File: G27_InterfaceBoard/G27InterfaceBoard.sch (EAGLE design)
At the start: 28 parts, among them IC1 LMV321M5, IC2 74HC126D, J1 Pedal, J2 Shifter, J3 Steering, U1 LMV324

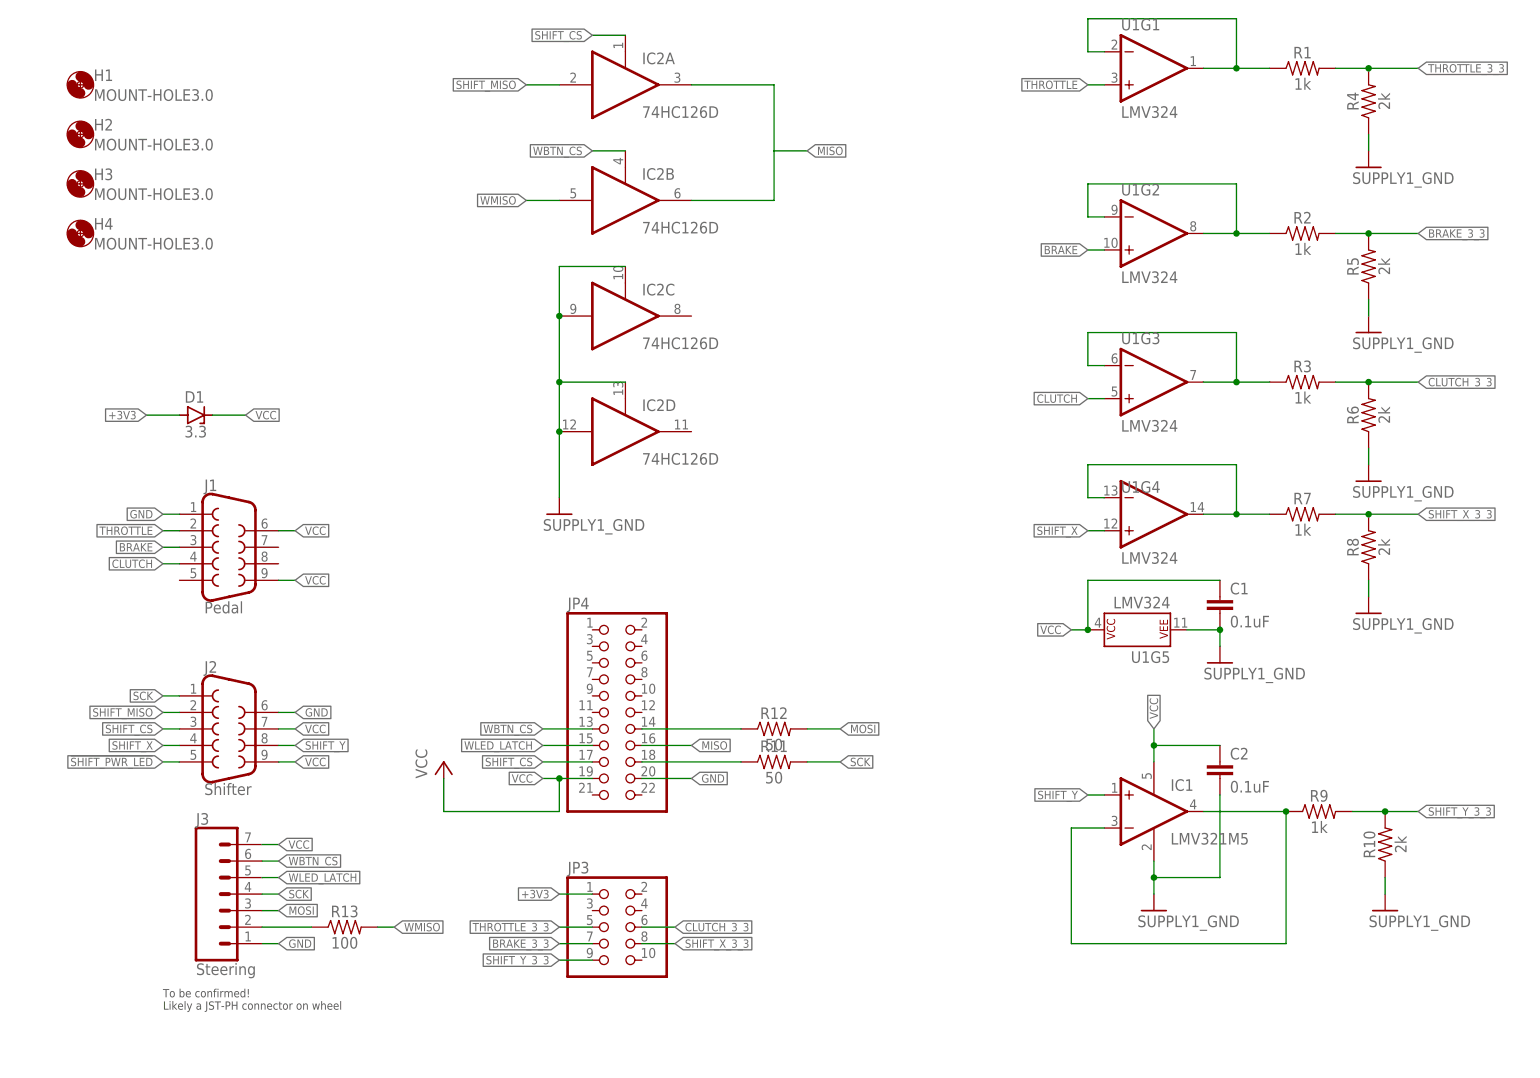
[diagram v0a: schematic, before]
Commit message: G27InterfaceBoard v1.0 as ordered.
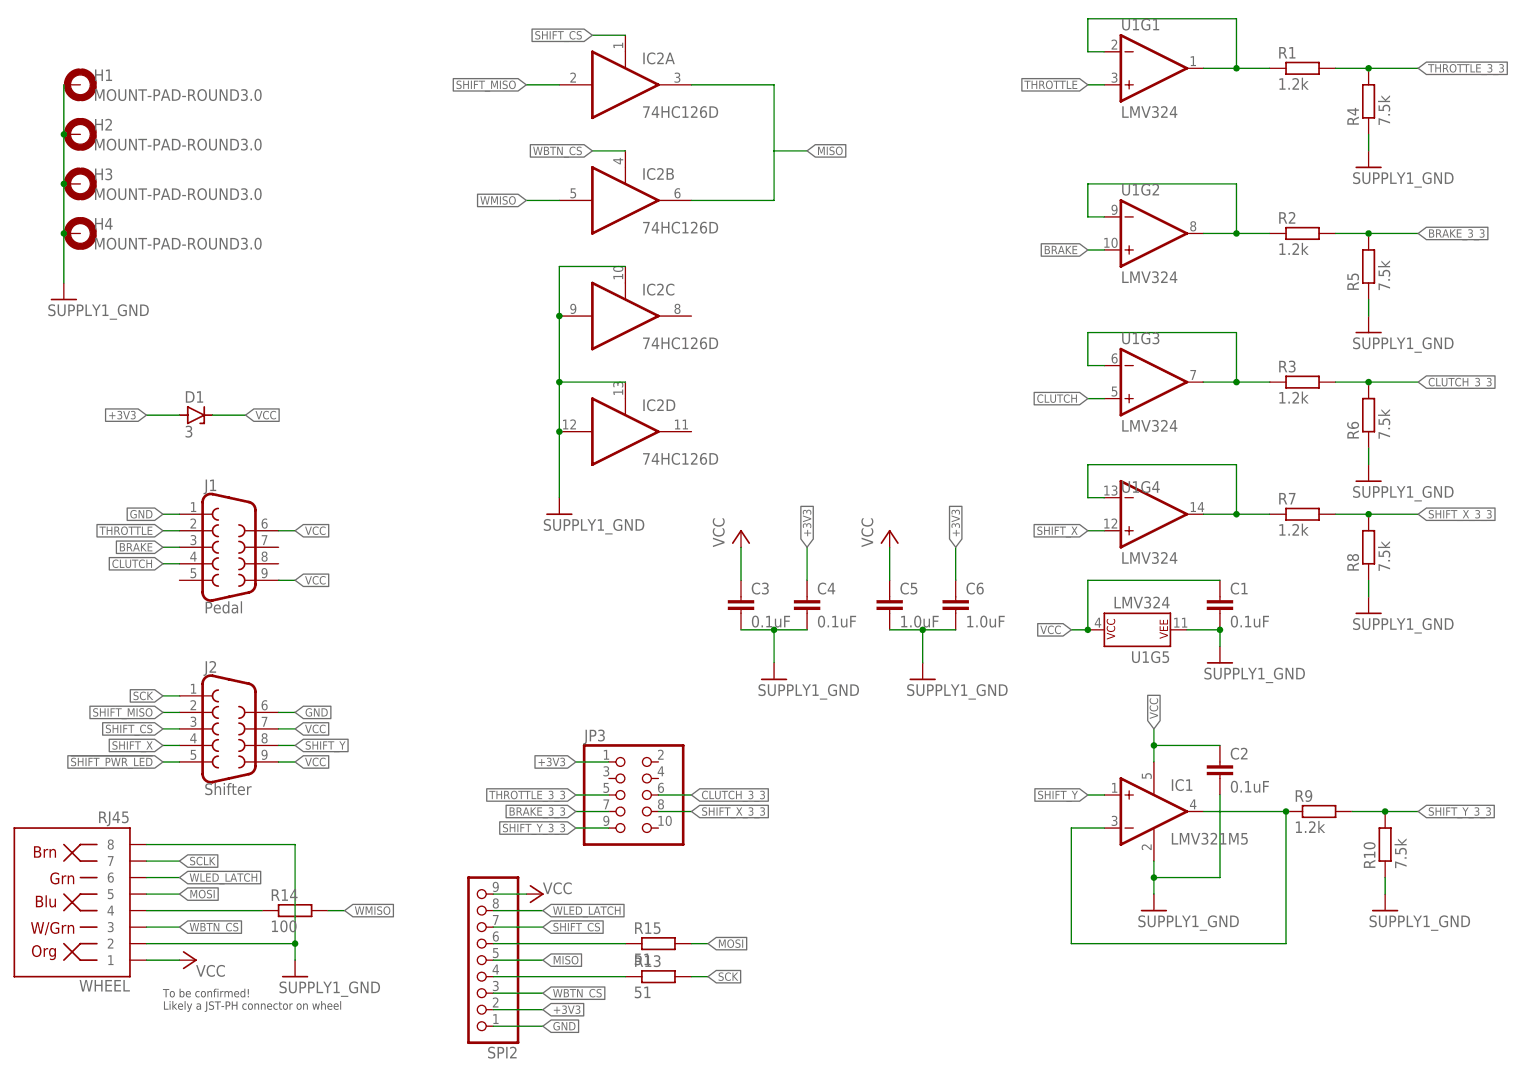
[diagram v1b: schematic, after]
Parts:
- removed J3: Steering, SparkFun-Connectors:CONN_07LONGPADS
- removed JP4: (no value), stm_board_f407:PINHEAD_PINHD-2X11
- removed R11, R12: 50, SparkFun-Resistors:RESISTOR0603
- added C3, C4: 0.1uF, resistor:C-EUC0805
- added C5, C6: 1.0uF, resistor:C-EUC0805
- added R14: 100, resistor:R-EU_R0603
- added R15: 51, resistor:R-EU_R0603
- added SPI2: (no value), pinhead:PINHD-1X9
- added WHEEL: RJ45, SparkFun-Connectors:RJ45-8
- D1: value 3.3 -> 3
- H1, H2, H3, H4: value MOUNT-HOLE3.0 -> MOUNT-PAD-ROUND3.0; device holes:MOUNT-HOLE3.0 -> holes:MOUNT-PAD-ROUND3.0
- R1, R2, R3, R7, R9: value 1k -> 1.2k; device SparkFun-Resistors:RESISTOR0603 -> resistor:R-EU_R0603
- R10, R4, R5, R6, R8: value 2k -> 7.5k; device SparkFun-Resistors:RESISTOR0603 -> resistor:R-EU_R0603
- R13: value 100 -> 51; device SparkFun-Resistors:RESISTOR0603 -> resistor:R-EU_R0603
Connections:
- removed net N$4: JP4.18, R11.1
- removed net N$7: JP4.14, R12.1
- new net N$10: R15.1, SPI2.6
- new net N$9: R14.1, WHEEL.4
- new net SCLK: WHEEL.7
- net +3V3: now also C4.1, C6.1, SPI2.2
- net GND: now also C3.2, C4.2, C5.2, C6.2, H1.MOUNT, H2.MOUNT, H3.MOUNT, H4.MOUNT, SPI2.1, WHEEL.2, WHEEL.8; no longer J3.1, JP4.20
- net MISO: now also SPI2.5; no longer JP4.16
- net MOSI: now also R15.2, WHEEL.5; no longer J3.3, R12.2
- net N$8: now also SPI2.4; no longer J3.2
- net SCK: now also R13.2; no longer J3.4, R11.2
- net SHIFT_CS: now also SPI2.7; no longer JP4.17
- net VCC: now also C3.1, C5.1, SPI2.9, WHEEL.1; no longer J3.7, JP4.19
- net WBTN_CS: now also SPI2.3, WHEEL.3; no longer J3.6, JP4.13
- net WLED_LATCH: now also SPI2.8, WHEEL.6; no longer J3.5, JP4.15
- net WMISO: now also R14.2; no longer R13.2
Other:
- moved on the sheet: JP3
